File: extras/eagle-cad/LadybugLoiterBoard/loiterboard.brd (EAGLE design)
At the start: 52.1 x 66.8 mm, 19 parts

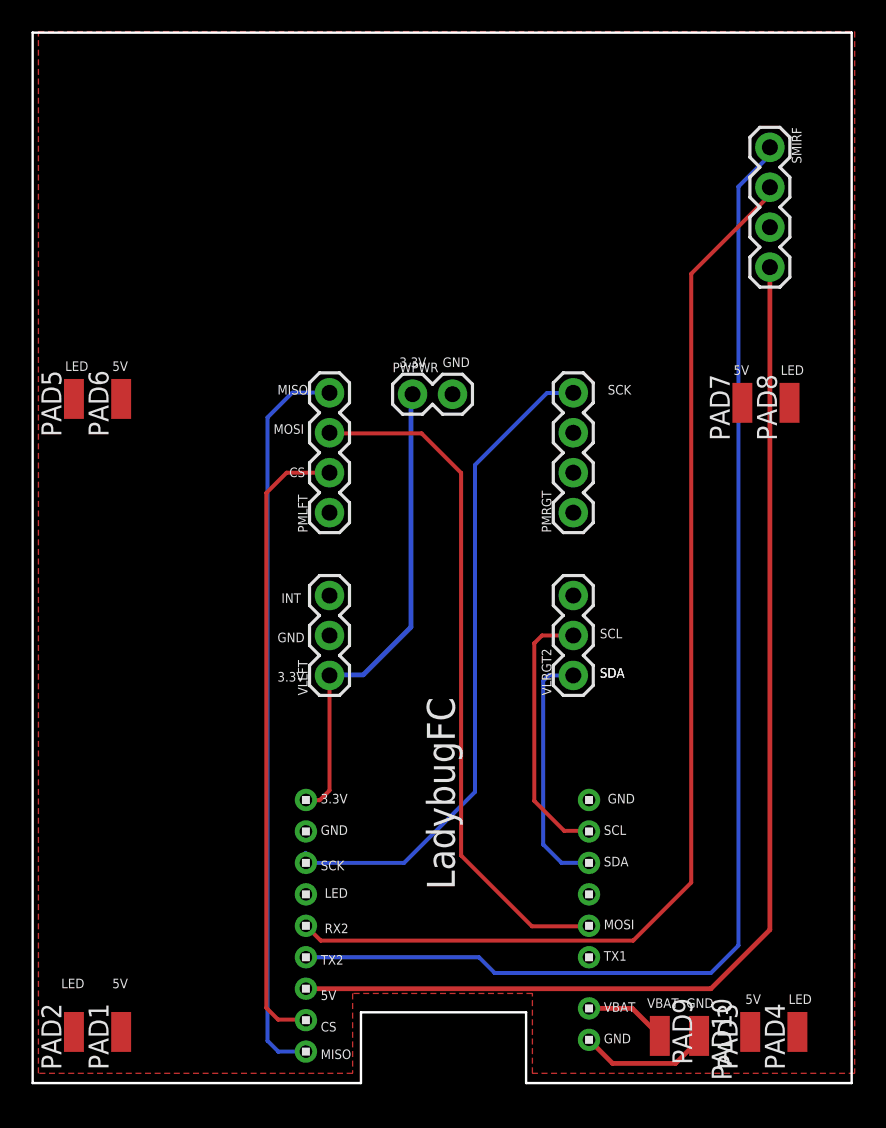
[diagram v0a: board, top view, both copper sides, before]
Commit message: More Ladybug Loiterboard work
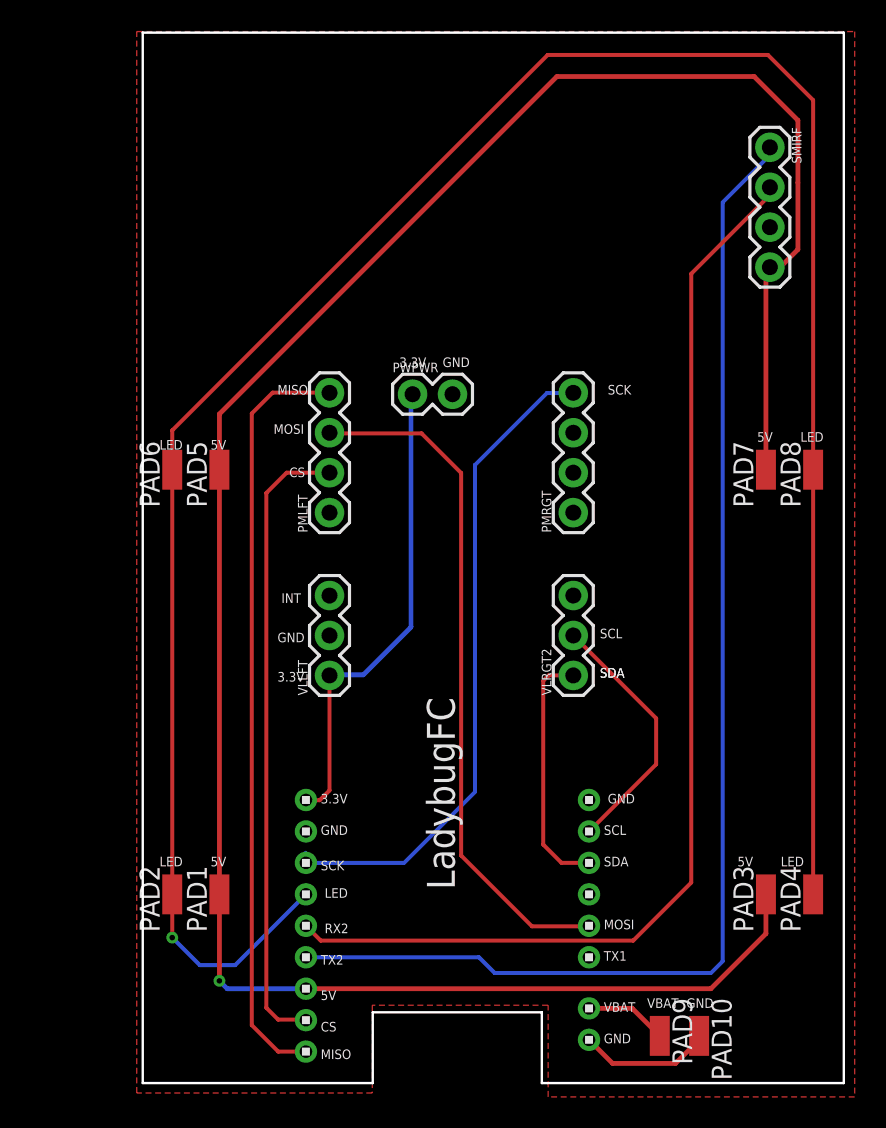
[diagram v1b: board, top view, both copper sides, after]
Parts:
- moved PAD1 10.8 mm to (15.0, 12.0)
- moved PAD2 10.8 mm to (12.0, 12.0)
- moved PAD5 10.3 mm to (15.0, 39.0)
- moved PAD3 8.81 mm to (49.8, 12.0)
- moved PAD4 8.81 mm to (52.8, 12.0)
- moved PAD6 5.55 mm to (12.0, 39.0)
- moved PAD7 4.51 mm to (49.8, 39.0)
- moved PAD8 4.51 mm to (52.8, 39.0)
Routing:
- net LED: track 0.00 -> 145.1 mm, vias 0 -> 1
- net 5V: track 72.7 -> 141.8 mm, vias 0 -> 1
- net D4/MISO: track 47.1 -> 48.5 mm, vias 0 -> 1
- net SCL: track 17.0 -> 16.4 mm
- net SDA: vias 0 -> 1
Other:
- board size 52.1 x 66.8 mm -> 44.6 x 66.8 mm
